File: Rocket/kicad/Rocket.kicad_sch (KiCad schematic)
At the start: 15 parts, among them Q1 Q_NPN_EBC, Q2 Q_NPN_EBC, U1 NE555P, U2 BAT_HLD_SMD

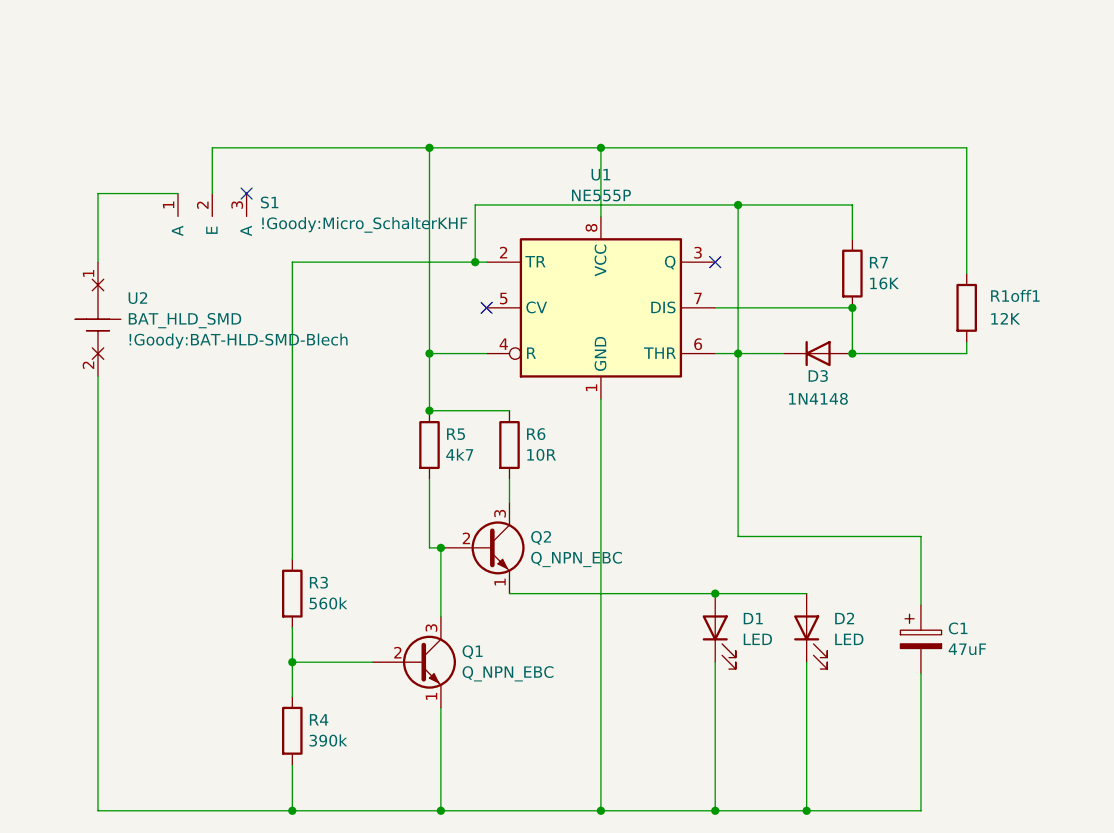
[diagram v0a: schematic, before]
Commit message: V08122025
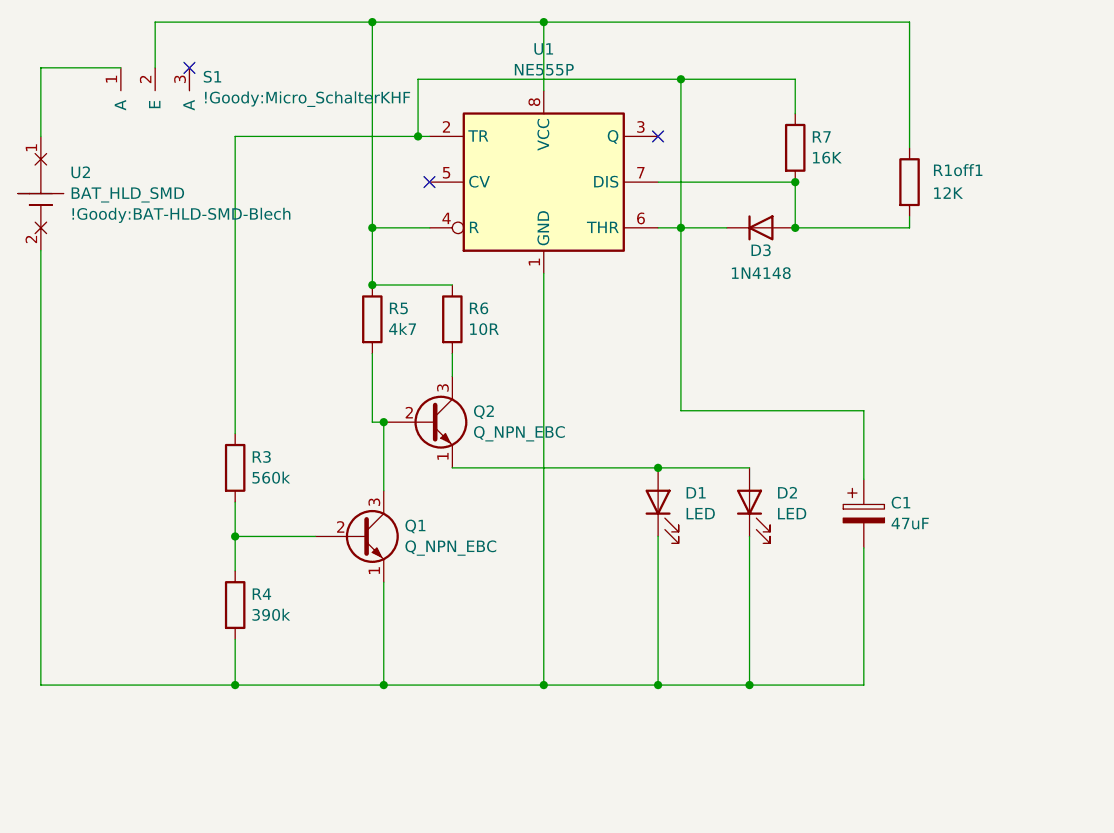
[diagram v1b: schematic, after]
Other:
- moved on the sheet: C1, D1, D2, D3, Q1, Q2, R1off1, R3, R4, R5, R6, R7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

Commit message: V10122025
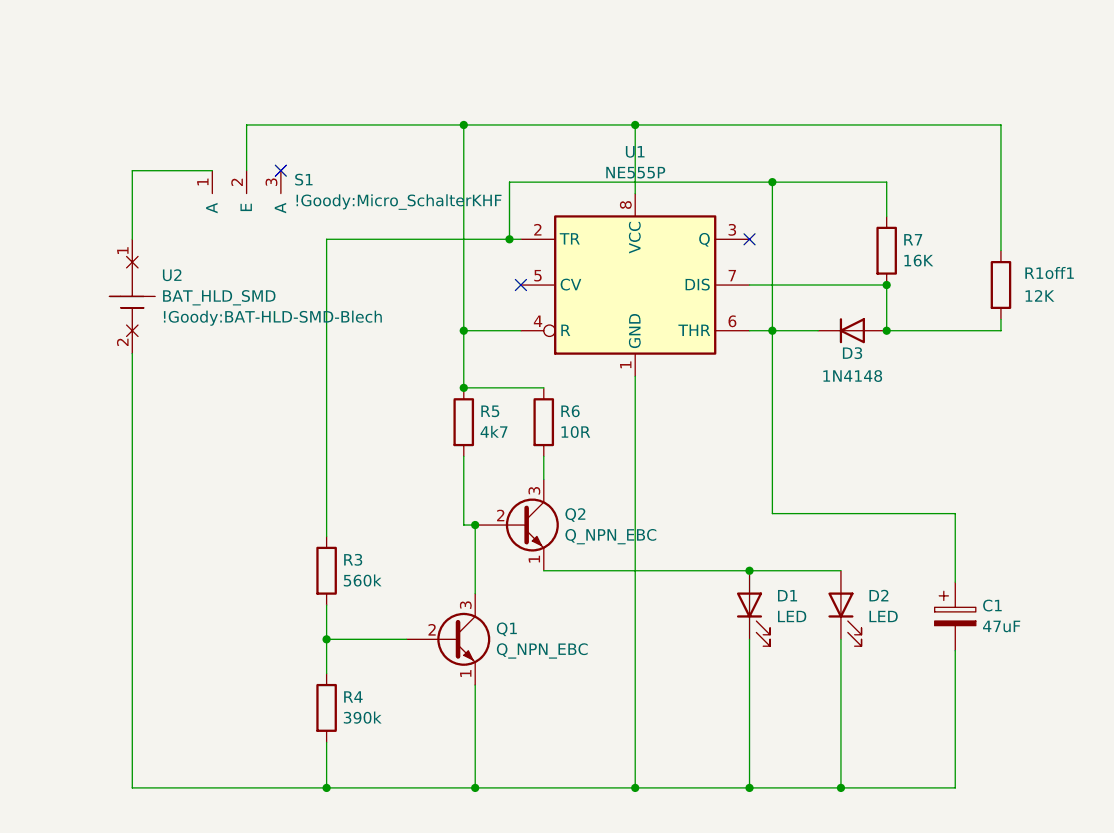
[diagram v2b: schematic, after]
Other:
- moved on the sheet: C1, D1, D2, D3, Q1, Q2, R1off1, R3, R4, R5, R6, R7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
